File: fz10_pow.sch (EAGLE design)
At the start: 82 parts

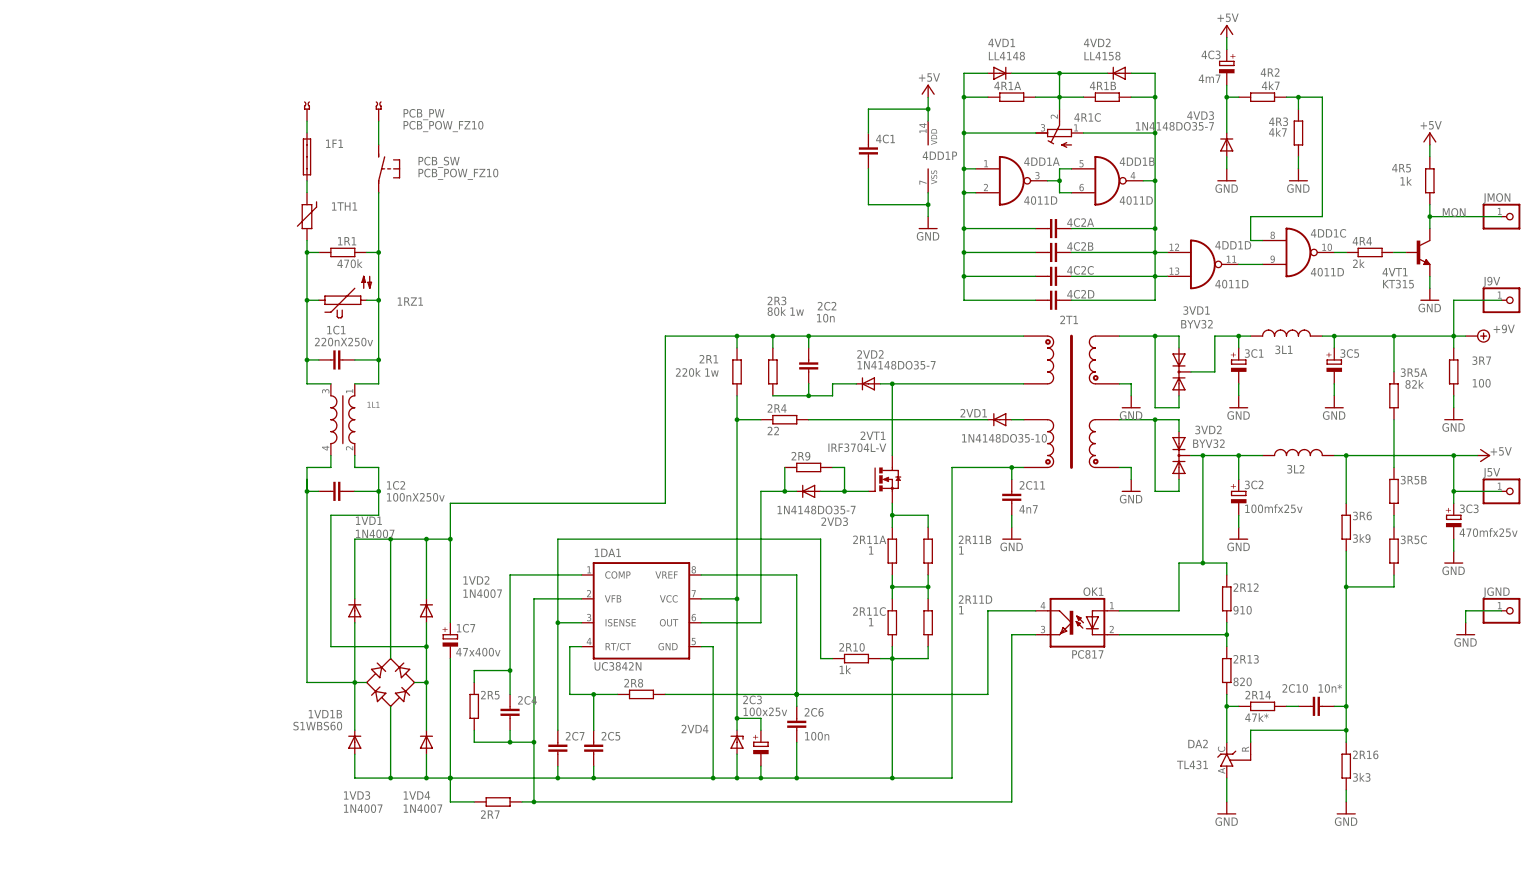
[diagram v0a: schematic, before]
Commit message: .
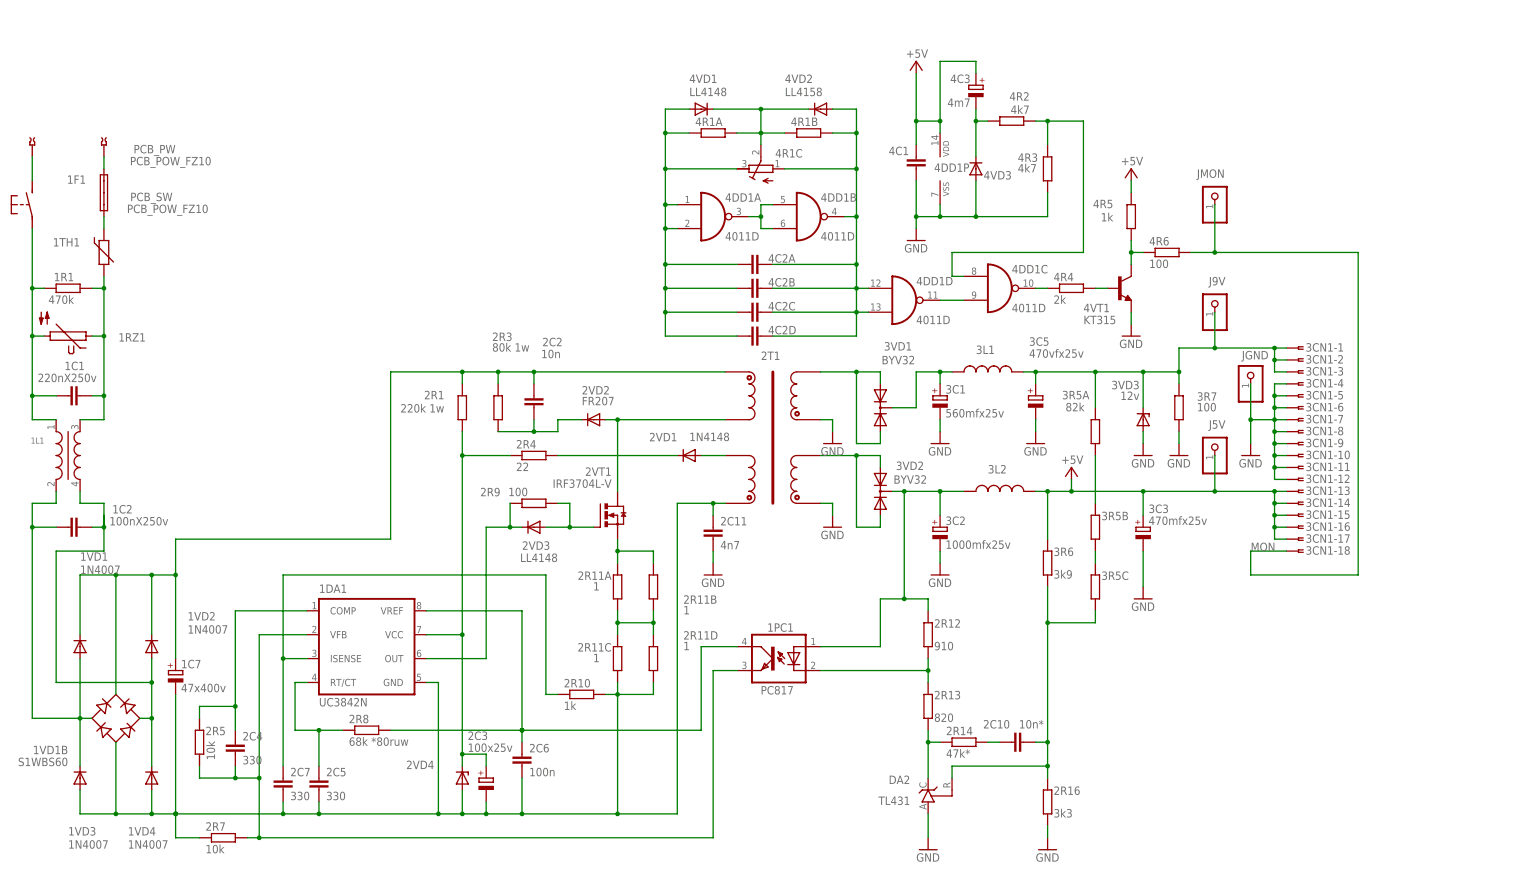
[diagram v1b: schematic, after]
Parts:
- removed OK1: PC817, optocoupler:PC817
- added 1PC1: PC817, optocoupler:PC817
- added 3CN1: (no value), 3do:FTOP-18
- added 3VD3: 12v, diode:ZENER-DIODEDO34-7
- added 4R6: 100, rcl:R-EU_M0805
- 1R1: device rcl:R-EU_0613/15 -> rcl:R-EU_0309/12
- 2C4, 2C5, 2C7: value (none) -> 330
- 2C6: device rcl:C-EUC1206 -> rcl:C-EUC0805
- 2R5: value (none) -> 10k; device rcl:R-EU_R1206 -> rcl:R-EU_M0805
- 2R7: value (none) -> 10k
- 2R8: value (none) -> 68k *80ruw
- 2R9: value (none) -> 100
- 2VD1: value 1N4148DO35-10 -> 1N4148
- 2VD2: value 1N4148DO35-7 -> FR207; device diode:1N4148DO35-7 -> diode:1N4148DO35-10
- 2VD3: value 1N4148DO35-7 -> LL4148; device diode:1N4148DO35-7 -> diode:DIODE-SOD80C
- 3C1: value (none) -> 560mfx25v
- 3C2: value 100mfx25v -> 1000mfx25v
- 3C5: value (none) -> 470vfx25v
- 4VD3: value 1N4148DO35-7 -> (none); device diode:1N4148DO35-7 -> diode:DIODE-SOD80C
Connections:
- removed net +9V: 3C5.+, 3L1.2, 3R5A.2, 3R7.2, J9V.1
- new net N$38: 3C5.+, 3CN1-1.1, 3CN1-2.1, 3CN1-3.1, 3L1.2, 3R5A.2, 3R7.2, 3VD3.C, J9V.1
- new net N$44: 1C2.1, 1L1.4, 1VD1B.AC1, 1VD2.A, 1VD4.C
- net +5V: now also 3CN1-13.1, 3CN1-14.1, 3CN1-15.1, 3CN1-16.1, 3CN1-17.1
- net GND: now also 2T1.9V2, 3CN1-10.1, 3CN1-11.1, 3CN1-12.1, 3CN1-4.1, 3CN1-5.1, 3CN1-6.1, 3CN1-7.1, 3CN1-8.1, 3CN1-9.1, 3VD3.A; no longer 2T1.O1.2
- net MON: now also 3CN1-18.1, 4R6.2; no longer 4R5.1, 4VT1.C
- net N$12: now also 1PC1.C; no longer OK1.C
- net N$13: now also 1PC1.A; no longer OK1.A
- net N$15: now also 1C2.2, 1L1.2; no longer 1C2.1, 1L1.4
- net N$20: now also 1PC1.COL; no longer OK1.COL
- net N$29: now also 4R5.1, 4R6.1, 4VT1.C; no longer 1C2.2, 1L1.2, 1VD1B.AC1, 1VD2.A, 1VD4.C
- net N$40: now also 1PC1.EMIT; no longer OK1.EMIT
- net N$5: now also 2T1.9V1; no longer 2T1.O1.1
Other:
- moved on the sheet: 1C1, 1C2, 1C7, 1DA1, 1F1, 1L1, 1R1, 1RZ1, 1TH1, 1VD1, 1VD1B, 1VD2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
